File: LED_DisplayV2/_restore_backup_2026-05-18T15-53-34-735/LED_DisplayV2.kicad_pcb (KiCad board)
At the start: 4 copper layers, 120 x 120 mm, 105 parts, among them U1 A3144, U10 AMS1117-5.0, U2 TPIC6C595N, U3 TPIC6C595N, U4 TPIC6C595N, U5 TPIC6C595N, U6 TPIC6C595N, U7 TPIC6C595N, U8 TPIC6C595N, U9 TPIC6C595N

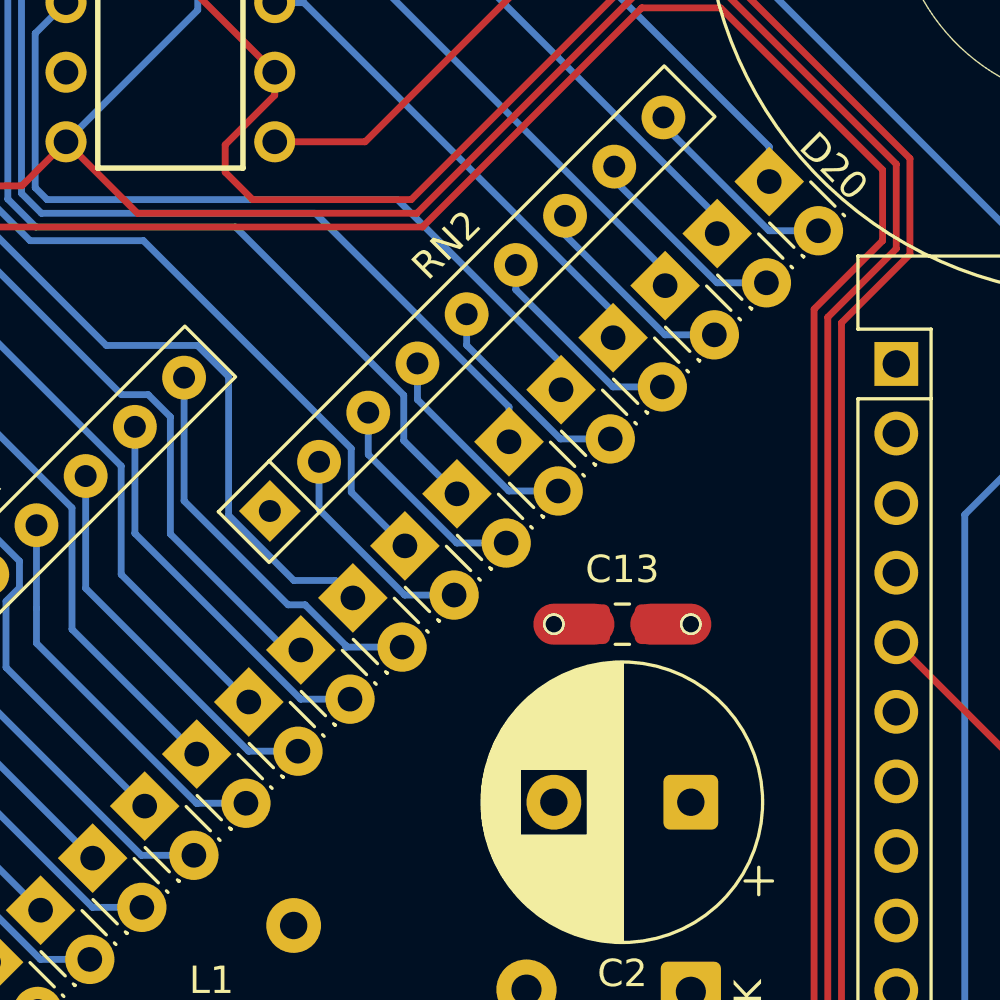
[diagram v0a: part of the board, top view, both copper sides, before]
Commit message: Fix1
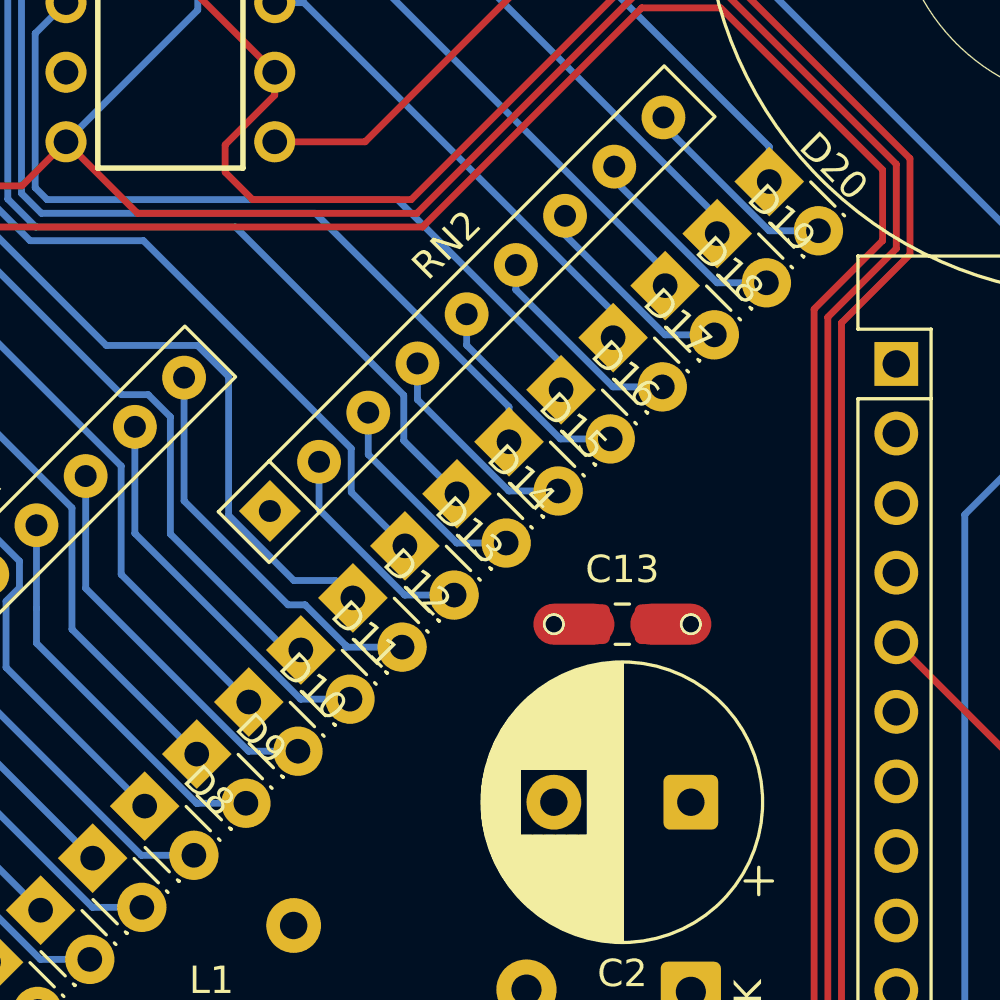
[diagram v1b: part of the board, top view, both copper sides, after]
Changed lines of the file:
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@@
 			(at 1.270001 -2.06 135)
 			(layer "F.SilkS")
-			(hide yes)
 			(effects
 				(font
@@
 			(at 1.270001 -2.06 135)
 			(layer "F.SilkS")
-			(hide yes)
 			(effects
 				(font
@@
 			(at 1.270001 -2.06 135)
 			(layer "F.SilkS")
-			(hide yes)
 			(effects
 				(font
@@
 			(at 1.270001 -2.06 135)
 			(layer "F.SilkS")
-			(hide yes)
 			(effects
 				(font
@@
 			(at 1.270001 -2.06 135)
 			(layer "F.SilkS")
-			(hide yes)
 			(effects
 				(font
@@
 			(at 1.270001 -2.06 135)
 			(layer "F.SilkS")
-			(hide yes)
 			(effects
 				(font
@@
 			(at 1.270001 -2.06 135)
 			(layer "F.SilkS")
-			(hide yes)
 			(effects
 				(font
@@
 			(at 1.270001 -2.06 135)
 			(layer "F.SilkS")
-			(hide yes)
 			(effects
 				(font
@@
 			(at 1.270001 -2.06 135)
 			(layer "F.SilkS")
-			(hide yes)
 			(effects
 				(font
@@
 			(at 1.270001 -2.06 135)
 			(layer "F.SilkS")
-			(hide yes)
 			(effects
 				(font
@@
 			(at 1.270001 -2.06 135)
 			(layer "F.SilkS")
-			(hide yes)
 			(effects
 				(font
@@
 			(at 1.270001 -2.06 135)
 			(layer "F.SilkS")
-			(hide yes)
 			(effects
 				(font
